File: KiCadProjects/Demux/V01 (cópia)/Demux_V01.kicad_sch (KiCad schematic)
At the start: 26 parts, among them J1 alimentacao analogica, J10 +3.3Vmux, J11 -9Vmux, J12 -5Vmux, J13 GNDmux, J14 conectorEletrodos, J15 conectorEletrodos, J2 sinais analogicos, J3 comunicacao / sinais digitais, J4 Conn_01x03, J5 Conn_01x02, J6 Conn_01x02, J7 Conn_01x02, J8 +9Vmux, J9 +5Vmux, U1A1 74HC4051, U1B1 74HC4051, U2 BluePill_STM32F103C, U2A2 74HC4051, U2B2 74HC4051, U3A3 74HC4051, U3B3 74HC4051, U4A4 74HC4051, U4B4 74HC4051, U5A1 74HC4051, U5B1 74HC4051

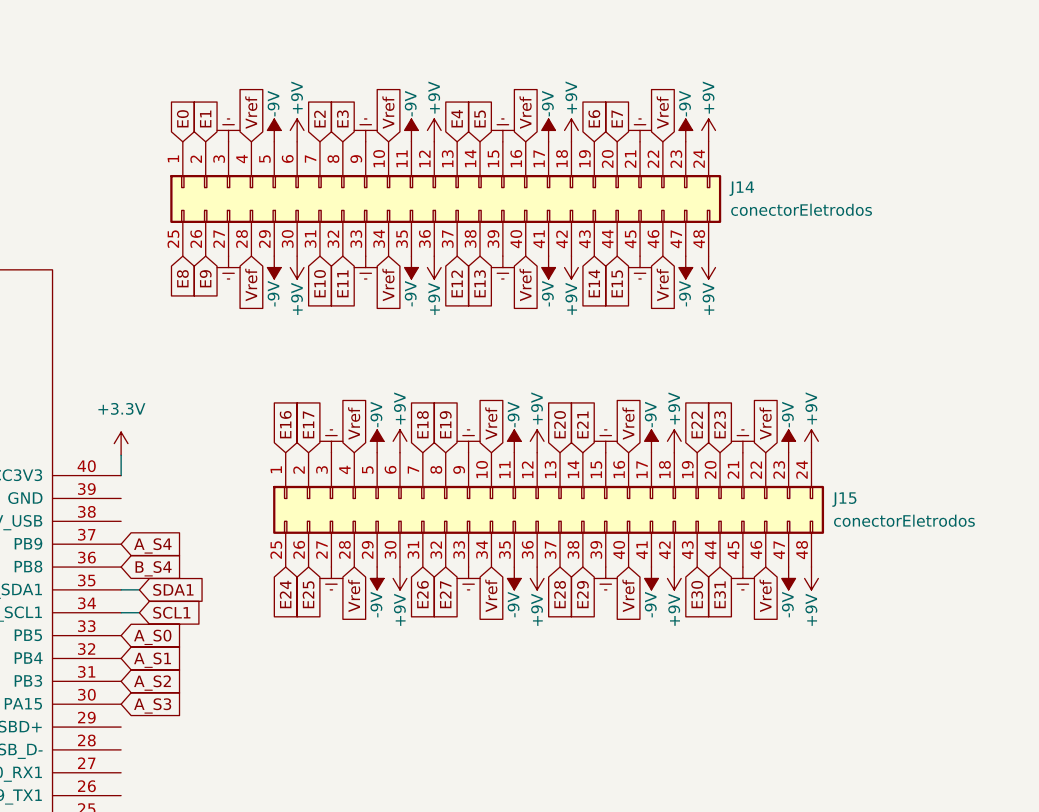
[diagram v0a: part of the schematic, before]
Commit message: tmp
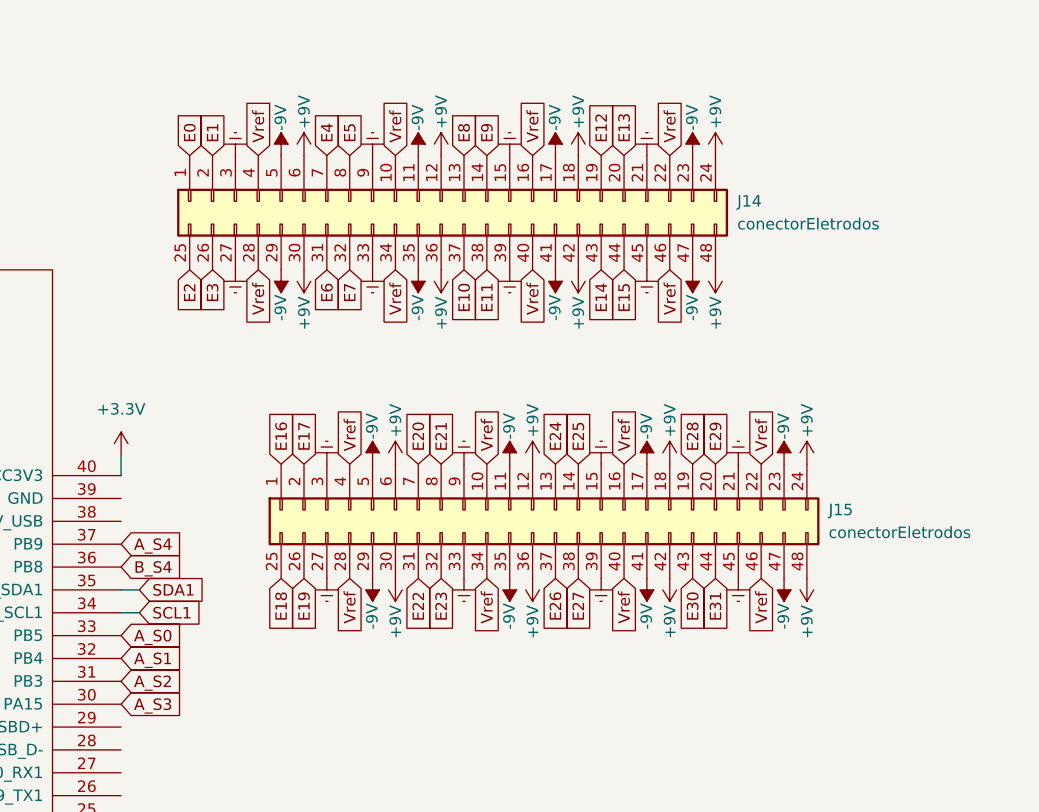
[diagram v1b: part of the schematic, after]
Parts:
- U1A1, U1B1, U2A2, U2B2, U3A3, U3B3, U4A4, U4B4, U5A1, U5B1: footprint HC4051:N16 -> 74HC4051N:N16
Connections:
- net E10: now also J14.37 (Pin_37); no longer J14.31 (Pin_31)
- net E11: now also J14.38 (Pin_38); no longer J14.32 (Pin_32)
- net E12: now also J14.19 (Pin_19); no longer J14.37 (Pin_37)
- net E13: now also J14.20 (Pin_20); no longer J14.38 (Pin_38)
- net E18: now also J15.25 (Pin_25); no longer J15.7 (Pin_7)
- net E19: now also J15.26 (Pin_26); no longer J15.8 (Pin_8)
- net E2: now also J14.25 (Pin_25); no longer J14.7 (Pin_7)
- net E20: now also J15.7 (Pin_7); no longer J15.13 (Pin_13)
- net E21: now also J15.8 (Pin_8); no longer J15.14 (Pin_14)
- net E22: now also J15.31 (Pin_31); no longer J15.19 (Pin_19)
- net E23: now also J15.32 (Pin_32); no longer J15.20 (Pin_20)
- net E24: now also J15.13 (Pin_13); no longer J15.25 (Pin_25)
- net E25: now also J15.14 (Pin_14); no longer J15.26 (Pin_26)
- net E26: now also J15.37 (Pin_37); no longer J15.31 (Pin_31)
- net E27: now also J15.38 (Pin_38); no longer J15.32 (Pin_32)
- net E28: now also J15.19 (Pin_19); no longer J15.37 (Pin_37)
- net E29: now also J15.20 (Pin_20); no longer J15.38 (Pin_38)
- net E3: now also J14.26 (Pin_26); no longer J14.8 (Pin_8)
- net E4: now also J14.7 (Pin_7); no longer J14.13 (Pin_13)
- net E5: now also J14.8 (Pin_8); no longer J14.14 (Pin_14)
- net E6: now also J14.31 (Pin_31); no longer J14.19 (Pin_19)
- net E7: now also J14.32 (Pin_32); no longer J14.20 (Pin_20)
- net E8: now also J14.13 (Pin_13); no longer J14.25 (Pin_25)
- net E9: now also J14.14 (Pin_14); no longer J14.26 (Pin_26)
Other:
- moved on the sheet: J14, J15
